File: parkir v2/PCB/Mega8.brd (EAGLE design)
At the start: 93 x 87 mm, 61 parts, among them IC1 ATMEGA8 (OR 168), IC2 DS1307, K1 ZF112, Q1 16000, T1 BC547, T2 BC557, T4 BC547

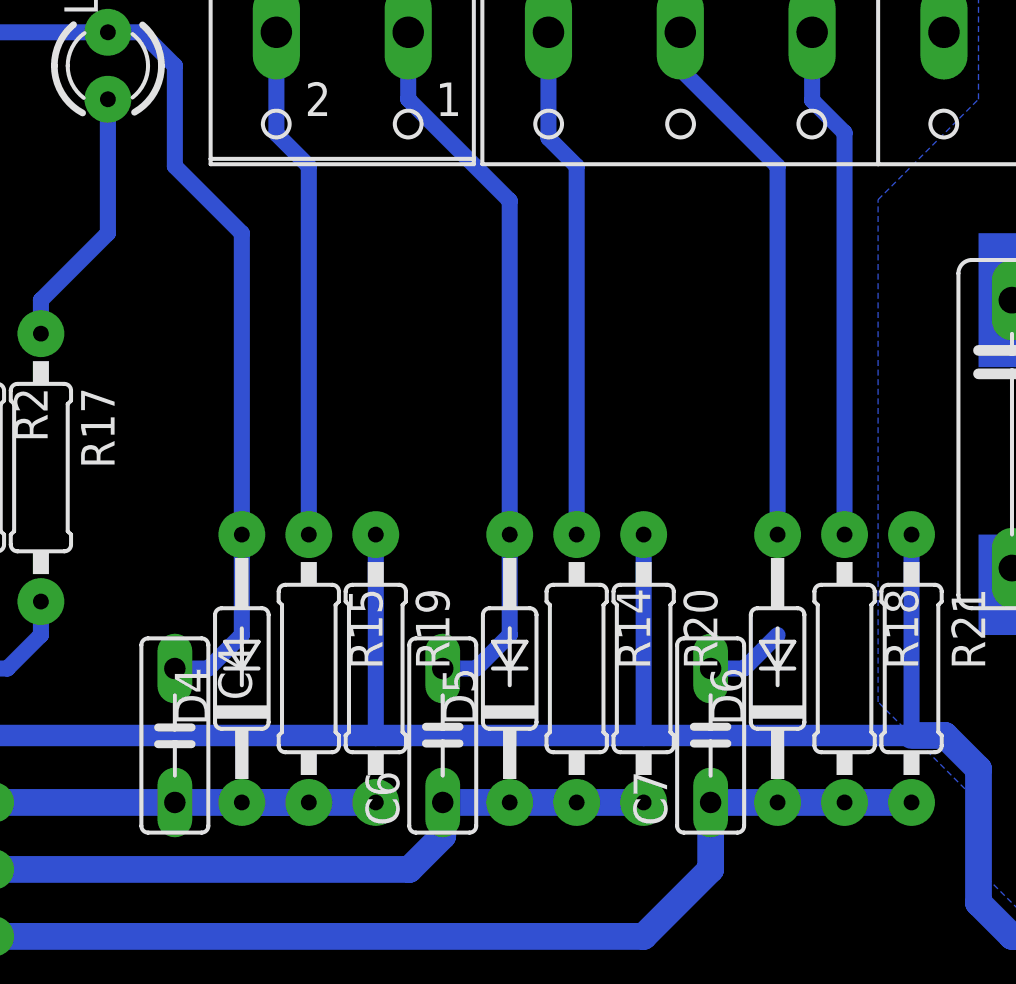
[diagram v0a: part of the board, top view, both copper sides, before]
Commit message: update pcb
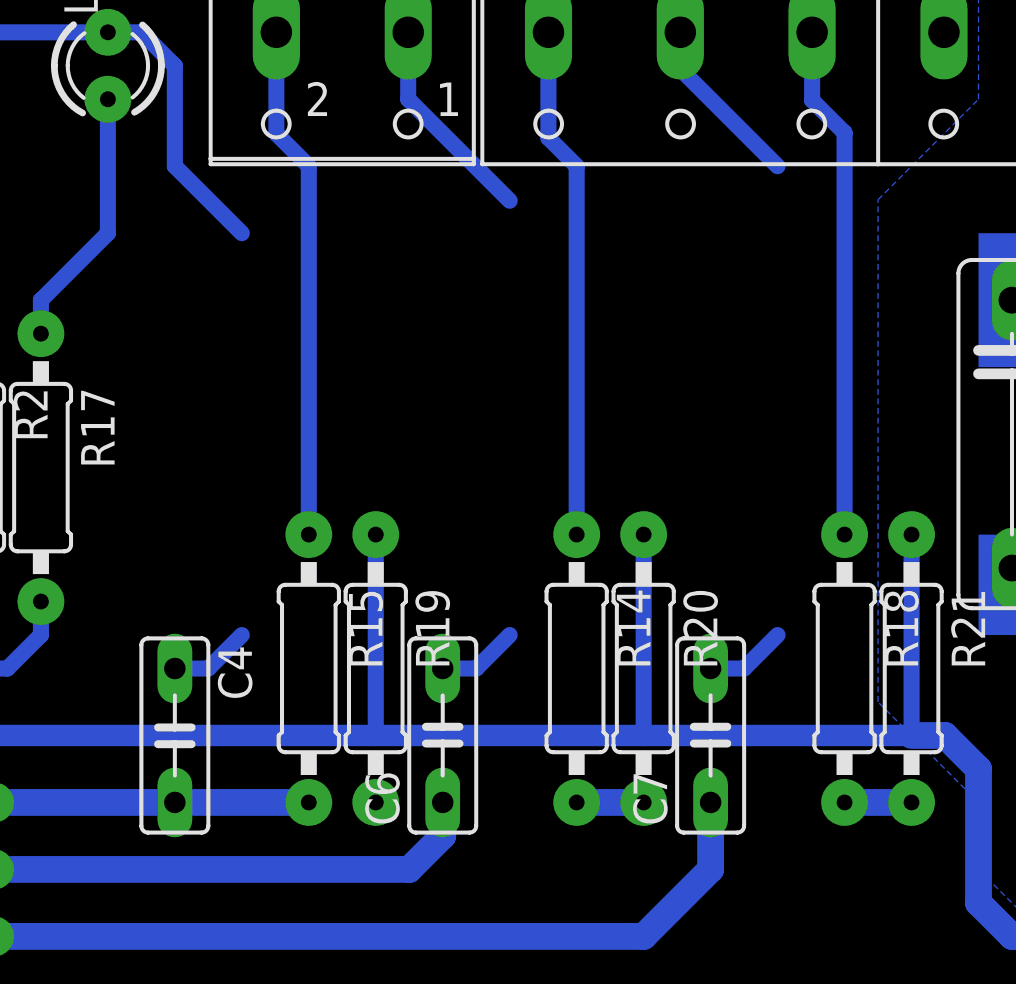
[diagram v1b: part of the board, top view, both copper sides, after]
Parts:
- removed D4, D5, D6: 1N4148, diode:DO35-10
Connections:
- net GND: no longer D4.A, D5.A, D6.A
- net N$13: no longer D4.C
- net N$14: no longer D5.C
- net N$20: no longer D6.C
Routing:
- net GND: track 591.3 -> 545.6 mm
- net N$13: track 20.3 -> 12.7 mm
- net N$20: track 39.2 -> 34.1 mm
- net N$14: track 27.2 -> 22.1 mm
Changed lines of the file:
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@@
 <element name="R18" library="rcl" package="0207/10" value="10k" x="64.77" y="58.42" rot="R270"/>
 <element name="C7" library="rcl" package="C050-025X075" value="100n" x="59.69" y="55.88" rot="R90"/>
-<element name="D4" library="diode" package="DO35-10" value="1N4148" x="41.91" y="58.42" rot="R90"/>
-<element name="D5" library="diode" package="DO35-10" value="1N4148" x="52.07" y="58.42" rot="R90"/>
-<element name="D6" library="diode" package="DO35-10" value="1N4148" x="62.23" y="58.42" rot="R90"/>
 <element name="R19" library="rcl" package="0207/10" value="10k" x="46.99" y="58.42" rot="R270"/>
 <element name="R20" library="rcl" package="0207/10" value="10k" x="57.15" y="58.42" rot="R270"/>
@@
 <contactref element="X4" pad="1"/>
 <contactref element="X4" pad="1"/>
-<contactref element="D6" pad="A"/>
-<contactref element="D5" pad="A"/>
-<contactref element="D4" pad="A"/>
 <wire x1="30.48" y1="82.55" x2="36.83" y2="82.55" width="0.6096" layer="16"/>
 <wire x1="48.22" y1="82.55" x2="48.22" y2="80.01" width="0.6096" layer="16"/>
@@
 <wire x1="39.37" y1="58.42" x2="40.64" y2="58.42" width="0.6096" layer="16"/>
 <wire x1="40.64" y1="58.42" x2="41.91" y2="59.69" width="0.6096" layer="16"/>
-<wire x1="41.91" y1="59.69" x2="41.91" y2="63.5" width="0.6096" layer="16"/>
-<wire x1="62.23" y1="63.5" x2="62.23" y2="77.47" width="0.6096" layer="16"/>
 <wire x1="62.23" y1="77.47" x2="58.42" y2="81.28" width="0.6096" layer="16"/>
 <wire x1="58.42" y1="81.28" x2="58.42" y2="82.43" width="0.6096" layer="16"/>
 <wire x1="58.42" y1="82.43" x2="58.54" y2="82.55" width="0.6096" layer="16"/>
-<wire x1="52.07" y1="63.5" x2="52.07" y2="76.16" width="0.6096" layer="16"/>
 <wire x1="52.07" y1="76.16" x2="48.22" y2="80.01" width="0.6096" layer="16"/>
 <wire x1="49.53" y1="58.42" x2="50.8" y2="58.42" width="0.6096" layer="16"/>
 <wire x1="50.8" y1="58.42" x2="52.07" y2="59.69" width="0.6096" layer="16"/>
-<wire x1="52.07" y1="59.69" x2="52.07" y2="63.5" width="0.6096" layer="16"/>
-<wire x1="41.91" y1="63.5" x2="41.91" y2="74.93" width="0.6096" layer="16"/>
 <wire x1="41.91" y1="74.93" x2="39.37" y2="77.47" width="0.6096" layer="16"/>
 <wire x1="39.37" y1="77.47" x2="39.37" y2="81.28" width="0.6096" layer="16"/>
 <wire x1="39.37" y1="81.28" x2="38.1" y2="82.55" width="0.6096" layer="16"/>
 <wire x1="38.1" y1="82.55" x2="36.83" y2="82.55" width="0.6096" layer="16"/>
+<wire x1="52.07" y1="59.69" x2="59.69" y2="58.42" width="0" layer="19" extent="16-16"/>
+<wire x1="41.91" y1="59.69" x2="49.53" y2="58.42" width="0" layer="19" extent="16-16"/>
+<wire x1="49.53" y1="43.18" x2="49.53" y2="58.42" width="0" layer="19" extent="1-1"/>
 </signal>
 <signal name="N$6">
@@
 <contactref element="IC1" pad="14"/>
 <contactref element="C4" pad="2"/>
-<contactref element="D4" pad="C"/>
 <contactref element="R19" pad="2"/>
 <wire x1="31.75" y1="53.34" x2="39.37" y2="53.34" width="1.016" layer="16"/>
 <wire x1="39.37" y1="53.34" x2="44.45" y2="53.34" width="1.016" layer="16"/>
-<wire x1="44.45" y1="53.34" x2="41.91" y2="53.34" width="1.016" layer="16"/>
-<wire x1="46.99" y1="53.34" x2="41.91" y2="53.34" width="1.016" layer="16"/>
+<wire x1="44.45" y1="53.34" x2="46.99" y2="53.34" width="0" layer="19" extent="1-1"/>
 </signal>
 <signal name="N$14">
@@
 <contactref element="R14" pad="2"/>
 <contactref element="C6" pad="1"/>
-<contactref element="D5" pad="C"/>
 <contactref element="R20" pad="2"/>
-<wire x1="49.53" y1="53.34" x2="52.07" y2="53.34" width="1.016" layer="16"/>
-<wire x1="52.07" y1="53.34" x2="54.61" y2="53.34" width="1.016" layer="16"/>
 <wire x1="54.61" y1="53.34" x2="57.15" y2="53.34" width="1.016" layer="16"/>
 <wire x1="49.53" y1="53.34" x2="49.53" y2="52.07" width="1.016" layer="16"/>
 <wire x1="49.53" y1="52.07" x2="48.26" y2="50.8" width="1.016" layer="16"/>
 <wire x1="48.26" y1="50.8" x2="31.75" y2="50.8" width="1.016" layer="16"/>
+<wire x1="49.53" y1="53.34" x2="54.61" y2="53.34" width="0" layer="19" extent="1-1"/>
 </signal>
 <signal name="N$16">
@@
 <contactref element="C7" pad="1"/>
 <contactref element="IC1" pad="12"/>
-<contactref element="D6" pad="C"/>
 <contactref element="R21" pad="2"/>
-<wire x1="59.69" y1="53.34" x2="62.23" y2="53.34" width="1.016" layer="16"/>
-<wire x1="62.23" y1="53.34" x2="64.77" y2="53.34" width="1.016" layer="16"/>
 <wire x1="64.77" y1="53.34" x2="67.31" y2="53.34" width="1.016" layer="16"/>
 <wire x1="59.69" y1="53.34" x2="59.69" y2="50.8" width="1.016" layer="16"/>
 <wire x1="59.69" y1="50.8" x2="57.15" y2="48.26" width="1.016" layer="16"/>
 <wire x1="57.15" y1="48.26" x2="31.75" y2="48.26" width="1.016" layer="16"/>
+<wire x1="59.69" y1="53.34" x2="64.77" y2="53.34" width="0" layer="19" extent="1-1"/>
 </signal>
 <signal name="N$5">
